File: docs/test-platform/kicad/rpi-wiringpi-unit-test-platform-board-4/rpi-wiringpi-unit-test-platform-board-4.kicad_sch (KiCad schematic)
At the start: 8 parts, among them J1 JST_IN_PWR, J2 JST_IN_I2C, M1 DS3231_0x68+AT24C32_0x57, M2 BMP180_0x77, M3 SSD1306_0x3c, SW1 SW_DIP_x01

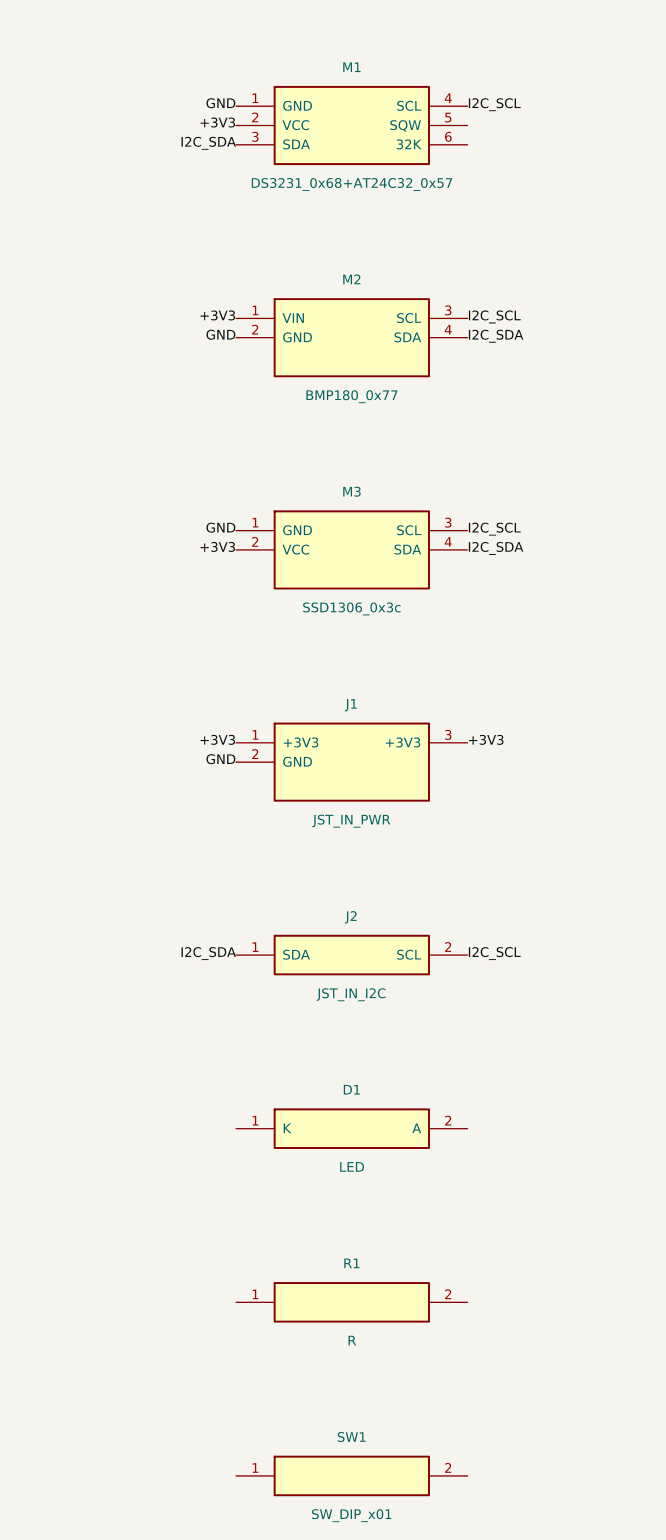
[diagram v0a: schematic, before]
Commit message: Updated boards
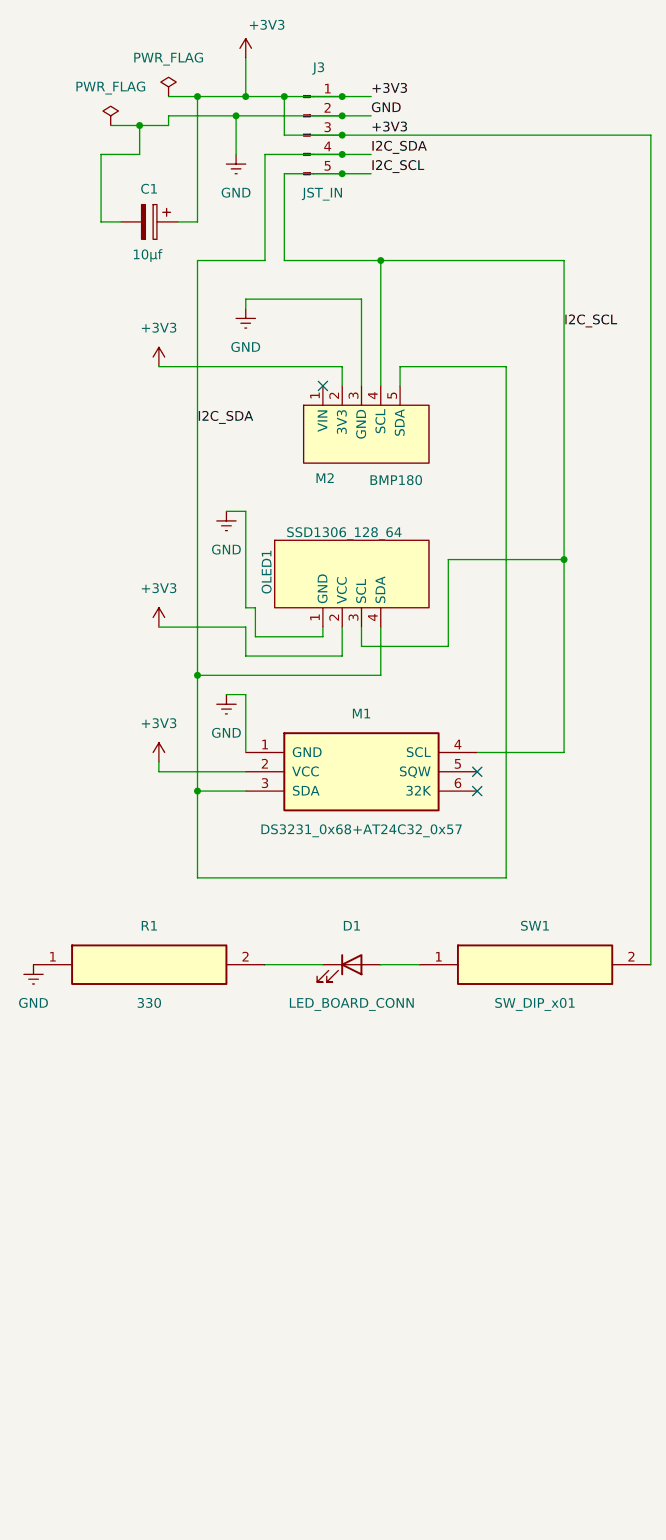
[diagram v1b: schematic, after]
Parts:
- removed J1: JST_IN_PWR, rpi-wiringpi-unit-test-platform-board-4:J1, symbol rpi-wiringpi-unit-test-platform-board-4:J1
- removed J2: JST_IN_I2C, rpi-wiringpi-unit-test-platform-board-4:J2, symbol rpi-wiringpi-unit-test-platform-board-4:J2
- removed M2: BMP180_0x77, rpi-wiringpi-unit-test-platform-board-4:M2, symbol rpi-wiringpi-unit-test-platform-board-4:M2
- removed M3: SSD1306_0x3c, rpi-wiringpi-unit-test-platform-board-4:M3, symbol rpi-wiringpi-unit-test-platform-board-4:M3
- added C1: 10µf, Capacitor_THT:CP_Radial_D5.0mm_P2.50mm, symbol Device:C_Polarized
- added J3: JST_IN, Connector_JST:JST_XH_B5B-XH-A_1x05_P2.50mm_Vertical, symbol Connector:Conn_01x05_Pin
- added M2: BMP180, RPi:BMP180, symbol RPi:BMP180
- added OLED1: SSD1306_128_64, RPi:OLED_SSD_1306_128_64, symbol RPi:OLED_SSD1306_128_64
- D1: value LED -> LED_BOARD_CONN; footprint rpi-wiringpi-unit-test-platform-board-4:D1 -> LED_THT:LED_D5.0mm; symbol rpi-wiringpi-unit-test-platform-board-4:D1 -> Device:LED
- R1: value R -> 330; footprint rpi-wiringpi-unit-test-platform-board-4:R1 -> Resistor_THT:R_Axial_DIN0207_L6.3mm_D2.5mm_P7.62mm_Horizontal
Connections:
- net +3V3: now also SW1.2, C1.1, J3.1 (Pin_1), J3.3 (Pin_3), M2.2 (3V3), OLED1.2 (VCC)
- net GND: now also R1.1, C1.2, J3.2 (Pin_2), M2.3 (GND), OLED1.1 (GND)
- net I2C_SCL: now also J3.5 (Pin_5), M2.4 (SCL), OLED1.3 (SCL)
- net I2C_SDA: now also J3.4 (Pin_4), M2.5 (SDA), OLED1.4 (SDA)
- net at R1.2: now also D1.1 (K)
- net at SW1.1: now also D1.2 (A)
- no-connect marks 0 -> 3
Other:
- moved on the sheet: M1, R1, SW1

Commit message: Finalize board 4 hardware
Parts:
- M1: footprint rpi-wiringpi-unit-test-platform-board-4:M1 -> RPi:DS3231
- SW1: footprint rpi-wiringpi-unit-test-platform-board-4:SW1 -> Button_Switch_SMD:SW_DIP_SPSTx01_Slide_6.7x4.1mm_W6.73mm_P2.54mm_LowProfile_JPin
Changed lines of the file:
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@@
 			)
 		)
-		(property "Footprint" "rpi-wiringpi-unit-test-platform-board-4:M1"
+		(property "Footprint" "RPi:DS3231"
 			(at 72.39 115.57 0)
 			(hide yes)
@@
 			)
 		)
-		(property "Footprint" "rpi-wiringpi-unit-test-platform-board-4:SW1"
+		(property "Footprint" "Button_Switch_SMD:SW_DIP_SPSTx01_Slide_6.7x4.1mm_W6.73mm_P2.54mm_LowProfile_JPin"
 			(at 95.25 140.97 0)
 			(hide yes)
